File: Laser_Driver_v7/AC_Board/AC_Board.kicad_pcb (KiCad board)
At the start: 2 copper layers, 62.4 x 42.7 mm, 9 parts, among them J1 Screw_Terminal_01x03, J2 Screw_Terminal_01x03, J3 Screw_Terminal_01x03

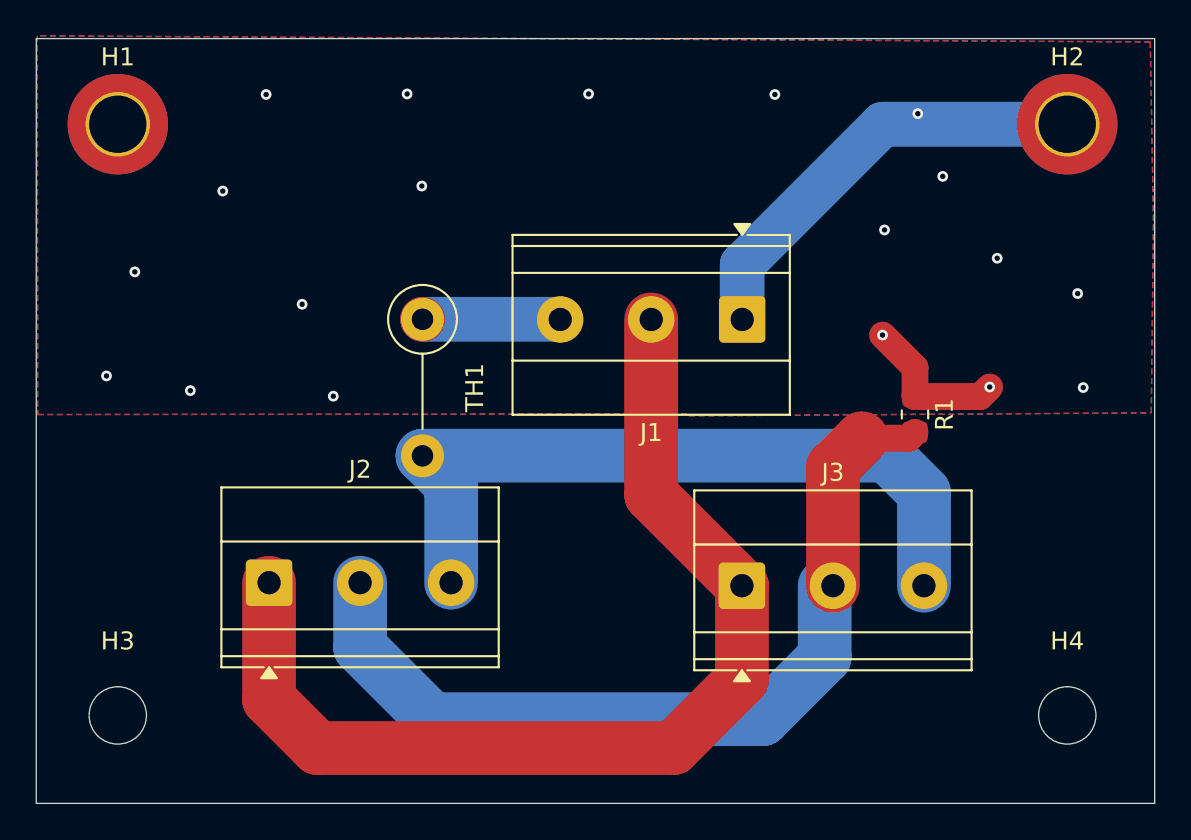
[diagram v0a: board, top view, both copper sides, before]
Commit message: Working towards a full set of pcbs in v7
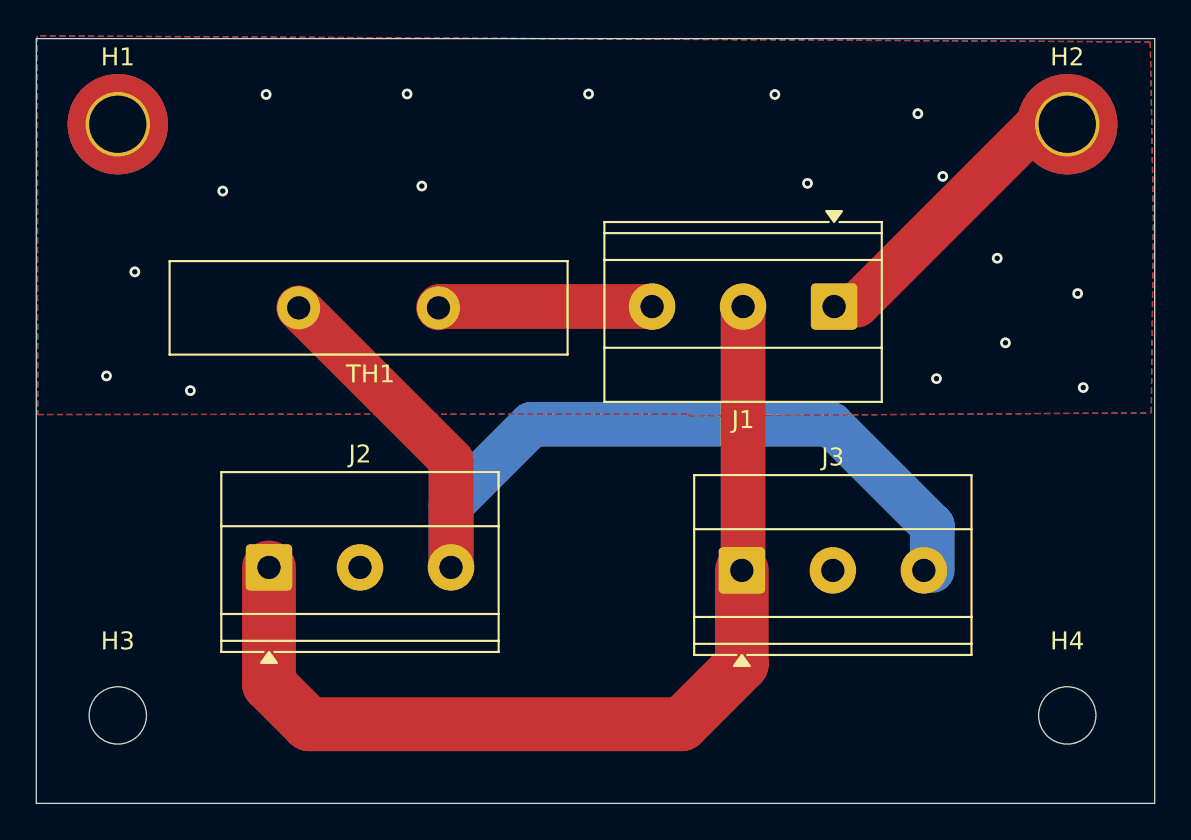
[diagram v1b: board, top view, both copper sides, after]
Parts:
- removed R1: 1k, Resistor_SMD:R_0805_2012Metric_Pad1.20x1.40mm_HandSolder
- TH1: footprint Resistor_THT:R_Axial_DIN0411_L9.9mm_D3.6mm_P7.62mm_Vertical -> Thermistor:Thermistor_Disc_D22.0mm_W5.0mm_P7.80mm_Ametherm_SL22
- moved J1 5.18 mm to (93.0, 50.2)
- moved TH1 1.10 mm to (70.9, 50.2), turned to 180 degrees
- moved J2 0.86 mm to (61.4, 64.7)
- moved J3 0.86 mm to (87.8, 64.9)
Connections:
- J2 pad 2: Net-(J2-Pin_2) -> unconnected-(J2-Pin_2-Pad2)
- J3 pad 2: Net-(J2-Pin_2) -> unconnected-(J3-Pin_2-Pad2)
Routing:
- net Net-(J2-Pin_2): track 48.6 -> 0.00 mm
- net Earth: track 33.0 -> 15.9 mm, vias 19 -> 17
- net /Line_TH: track 41.8 -> 55.1 mm
- net 120Vac: track 7.70 -> 12.0 mm
- net Neutral: track 57.8 -> 55.2 mm
